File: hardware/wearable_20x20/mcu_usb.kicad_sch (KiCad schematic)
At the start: 9 parts, among them U10 ESP32-S3FN8, U11 USBLC6-2SC6, Y1 L327S400H11L 40MHz 10pF

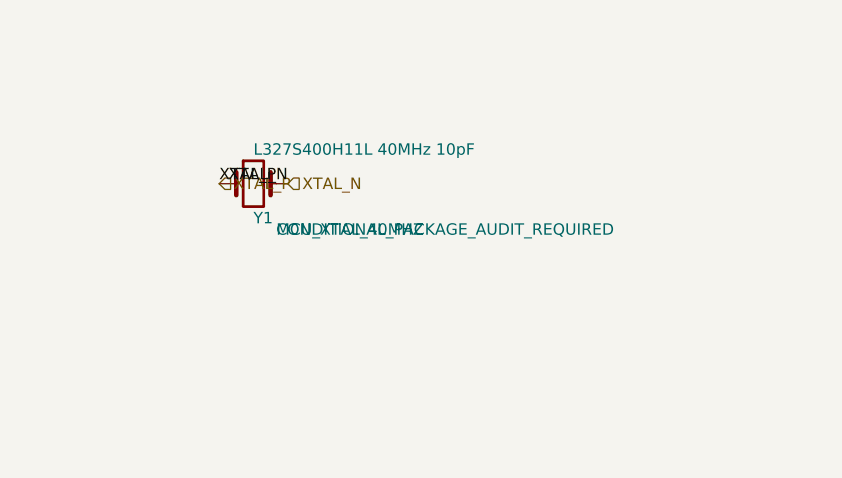
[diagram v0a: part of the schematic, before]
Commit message: Release crystal and power inductor packages
Co-authored-by: illiapliukhin <illiapliukhin@users.noreply.github.com>
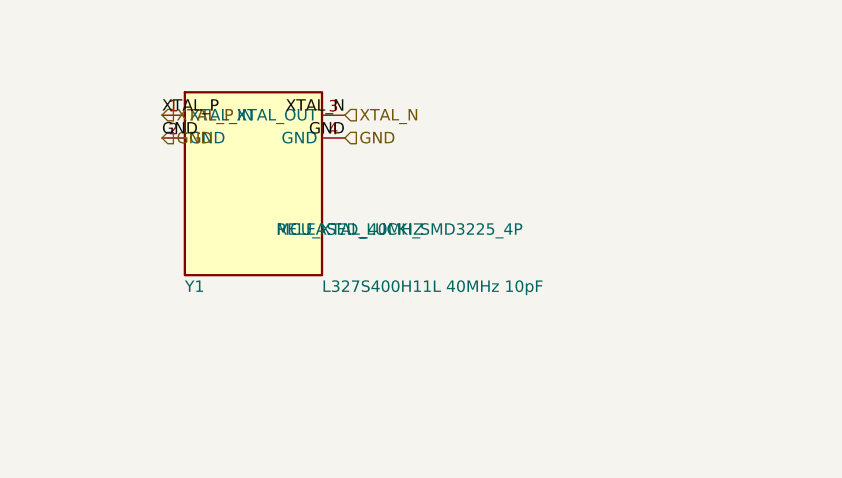
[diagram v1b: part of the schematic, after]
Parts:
- Y1: footprint (none) -> PartSignal_Packages:Lucki_L327S400H11L_Crystal_3225-4Pin; symbol Device:Crystal -> PartSignal_Platform:L327S400H11L; FootprintStatus CONDITIONAL_PACKAGE_AUDIT_REQUIRED -> RELEASED_LUCKI_SMD3225_4P
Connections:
- net GND: now also Y1.2 (GND), Y1.4 (GND)
- net XTAL_N: now also Y1.3 (XTAL_OUT); no longer Y1.2
